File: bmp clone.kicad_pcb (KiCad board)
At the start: 2 copper layers, 55 x 31 mm, 41 parts, among them J1 Conn_02x10_Odd_Even, J2 USB_B_Mini, J3 Jumper_2_Open, Q1 BC846, U1 STM32F103RBTx, U2 USBLC6-2P6, U3 TXS0108EPW, U4 AMS1117-3.3, X1 8MHz

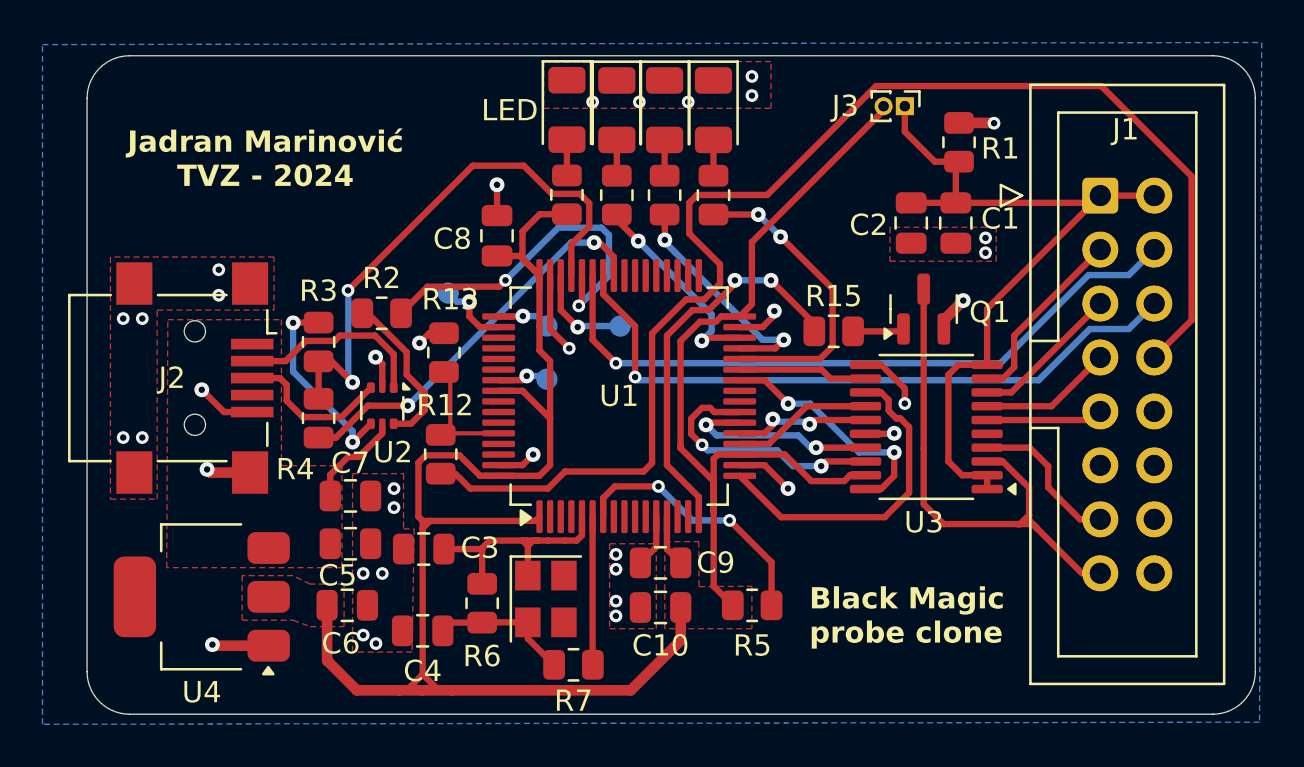
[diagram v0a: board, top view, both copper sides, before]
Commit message: manje dorade
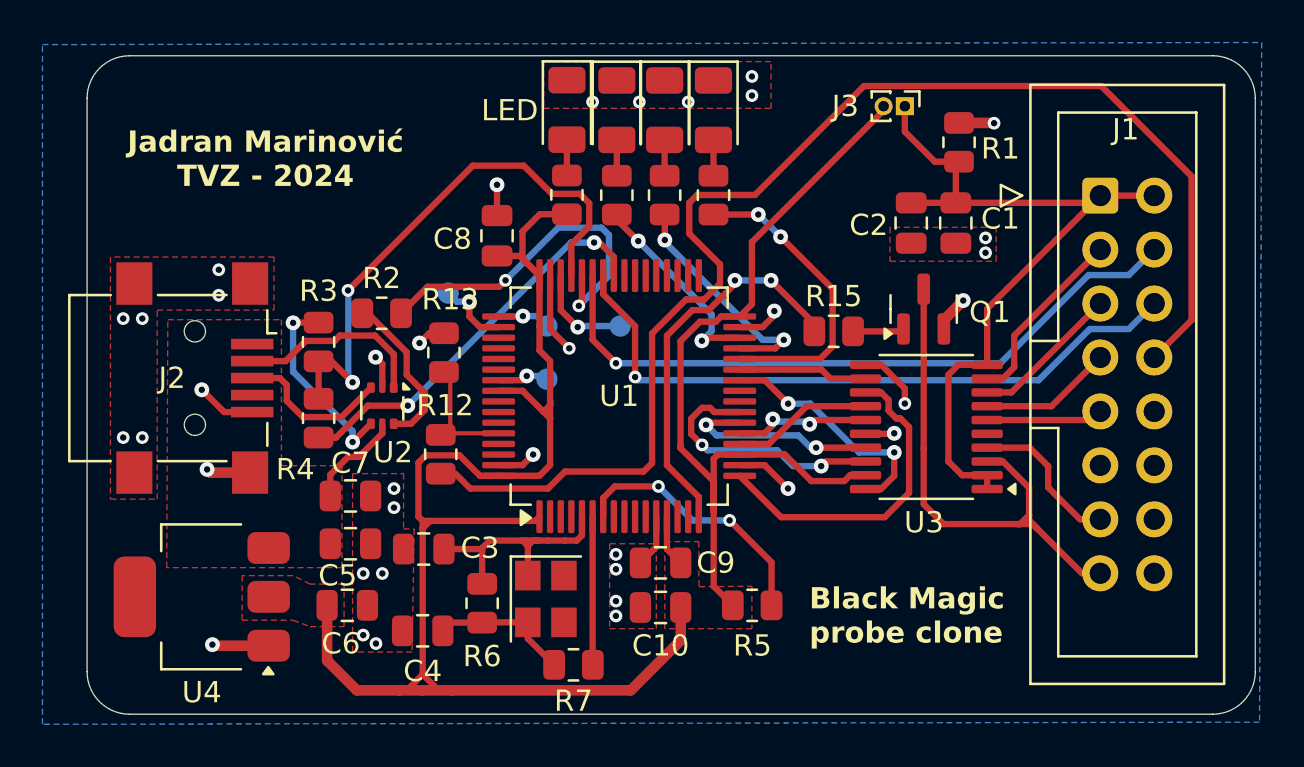
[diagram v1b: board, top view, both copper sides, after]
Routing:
- net +3.3V: track 110.3 -> 110.9 mm
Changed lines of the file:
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@@
-	)
-	(segment
-		(start 134.2 92.8)
-		(end 132.9 91.5)
-		(width 0.3)
-		(layer "F.Cu")
-		(net 6)
 	)
 	(segment
@@
 	)
 	(segment
+		(start 134.2 92.175)
+		(end 134.2 91.975)
+		(width 0.3)
+		(layer "F.Cu")
+		(net 6)
+	)
+	(segment
 		(start 140.339852 94.2)
 		(end 141.9 95.760148)
@@
 		(start 143.125 94.5)
 		(end 145.25 94.5)
+		(width 0.3)
+		(layer "F.Cu")
+		(net 6)
+	)
+	(segment
+		(start 134.2 92.8)
+		(end 133.8875 92.4875)
 		(width 0.3)
 		(layer "F.Cu")
@@
 	)
 	(segment
+		(start 133.8875 92.4875)
+		(end 134.2 92.175)
+		(width 0.3)
+		(layer "F.Cu")
+		(net 6)
+	)
+	(segment
 		(start 134.2 90.1)
 		(end 133.7 89.6)
@@
 	)
 	(segment
+		(start 134.2 92.8)
+		(end 134.2 91.975)
+		(width 0.3)
+		(layer "F.Cu")
+		(net 6)
+	)
+	(segment
 		(start 123.7 104.2)
 		(end 123.7 101.6)
@@
 	)
 	(segment
+		(start 133.8875 92.4875)
+		(end 132.9 91.5)
+		(width 0.3)
+		(layer "F.Cu")
+		(net 6)
+	)
+	(segment
 		(start 128.2 98)
 		(end 128.2 97.975)
@@
 	)
 	(segment
-		(start 134.2 92.8)
-		(end 134.2 90.1)
-		(width 0.3)
-		(layer "F.Cu")
-		(net 6)
-	)
-	(segment
 		(start 128.344544 94.5375)
 		(end 129.93438 94.5375)
@@
 		(start 133.7 95.5)
 		(end 134.2 95)
+		(width 0.3)
+		(layer "F.Cu")
+		(net 6)
+	)
+	(segment
+		(start 134.2 91.975)
+		(end 134.2 90.1)
 		(width 0.3)
 		(layer "F.Cu")
@@
 	)
 	(segment
-		(start 144.42 82.28)
-		(end 149.55 77.15)
+		(start 130.4375 96.1)
+		(end 134.1 96.1)
+		(width 0.3)
+		(layer "F.Cu")
+		(net 14)
+	)
+	(segment
+		(start 142.2 86.45312)
+		(end 142.2 85.55)
+		(width 0.3)
+		(layer "F.Cu")
+		(net 14)
+	)
+	(segment
+		(start 134.9 95.3)
+		(end 138.6 95.3)
+		(width 0.3)
+		(layer "F.Cu")
+		(net 14)
+	)
+	(segment
+		(start 139 88.8)
+		(end 140.6 87.2)
+		(width 0.3)
+		(layer "F.Cu")
+		(net 14)
+	)
+	(segment
+		(start 140.75 84.1)
+		(end 140.75 82.65)
 		(width 0.3)
 		(layer "F.Cu")
@@
 	)
 	(segment
+		(start 160.15 77.15)
+		(end 164.4 81.4)
+		(width 0.3)
+		(layer "F.Cu")
+		(net 14)
+	)
+	(segment
+		(start 141.45312 87.2)
+		(end 142.2 86.45312)
+		(width 0.3)
+		(layer "F.Cu")
+		(net 14)
+	)
+	(segment
+		(start 143.845 82.28)
+		(end 148.975 77.15)
+		(width 0.3)
+		(layer "F.Cu")
+		(net 14)
+	)
+	(segment
+		(start 129.75 95.4125)
+		(end 130.4375 96.1)
+		(width 0.3)
+		(layer "F.Cu")
+		(net 14)
+	)
+	(segment
+		(start 134.1 96.1)
+		(end 134.9 95.3)
+		(width 0.3)
+		(layer "F.Cu")
+		(net 14)
+	)
+	(segment
+		(start 142.2 85.55)
+		(end 140.75 84.1)
+		(width 0.3)
+		(layer "F.Cu")
+		(net 14)
+	)
+	(segment
+		(start 148.975 77.15)
+		(end 160.15 77.15)
+		(width 0.3)
+		(layer "F.Cu")
+		(net 14)
+	)
+	(segment
+		(start 164.4 81.4)
+		(end 164.4 88.1725)
+		(width 0.3)
+		(layer "F.Cu")
+		(net 14)
+	)
+	(segment
+		(start 140.6 87.2)
+		(end 141.45312 87.2)
+		(width 0.3)
+		(layer "F.Cu")
+		(net 14)
+	)
+	(segment
+		(start 140.75 82.65)
+		(end 141.12 82.28)
+		(width 0.3)
+		(layer "F.Cu")
+		(net 14)
+	)
+	(segment
 		(start 138.6 95.3)
 		(end 139 94.9)
@@
 	)
 	(segment
-		(start 129.75 95.4125)
-		(end 130.4375 96.1)
-		(width 0.3)
-		(layer "F.Cu")
-		(net 14)
-	)
-	(segment
-		(start 140.75 84.1)
-		(end 140.75 82.65)
-		(width 0.3)
-		(layer "F.Cu")
-		(net 14)
-	)
-	(segment
-		(start 134.9 95.3)
-		(end 138.6 95.3)
-		(width 0.3)
-		(layer "F.Cu")
-		(net 14)
-	)
-	(segment
-		(start 164.4 81.4)
-		(end 164.4 88.1725)
-		(width 0.3)
-		(layer "F.Cu")
-		(net 14)
-	)
-	(segment
-		(start 134.1 96.1)
-		(end 134.9 95.3)
-		(width 0.3)
-		(layer "F.Cu")
-		(net 14)
-	)
-	(segment
-		(start 141.45312 87.2)
-		(end 142.2 86.45312)
-		(width 0.3)
-		(layer "F.Cu")
-		(net 14)
-	)
-	(segment
-		(start 140.6 87.2)
-		(end 141.45312 87.2)
-		(width 0.3)
-		(layer "F.Cu")
-		(net 14)
-	)
-	(segment
-		(start 130.4375 96.1)
-		(end 134.1 96.1)
-		(width 0.3)
-		(layer "F.Cu")
-		(net 14)
-	)
-	(segment
-		(start 142.2 85.55)
-		(end 140.75 84.1)
-		(width 0.3)
-		(layer "F.Cu")
-		(net 14)
-	)
-	(segment
-		(start 160.15 77.15)
-		(end 164.4 81.4)
-		(width 0.3)
-		(layer "F.Cu")
-		(net 14)
-	)
-	(segment
-		(start 141.12 82.28)
-		(end 144.42 82.28)
-		(width 0.3)
-		(layer "F.Cu")
-		(net 14)
-	)
-	(segment
 		(start 164.4 88.1725)
 		(end 162.6425 89.93)
@@
 	)
 	(segment
-		(start 140.75 82.65)
-		(end 141.12 82.28)
-		(width 0.3)
-		(layer "F.Cu")
-		(net 14)
-	)
-	(segment
-		(start 142.2 86.45312)
-		(end 142.2 85.55)
-		(width 0.3)
-		(layer "F.Cu")
-		(net 14)
-	)
-	(segment
-		(start 149.55 77.15)
-		(end 160.15 77.15)
-		(width 0.3)
-		(layer "F.Cu")
-		(net 14)
-	)
-	(segment
-		(start 139 88.8)
-		(end 140.6 87.2)
-		(width 0.3)
-		(layer "F.Cu")
+		(start 141.12 82.28)
+		(end 143.845 82.28)
+		(width 0.3)
+		(layer "F.Cu")
